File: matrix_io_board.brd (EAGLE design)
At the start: 155.7 x 37.8 mm, 118 parts, among them IC1 6N138, IC10 REG1117, IC12 AP3012, IC2 SN74LVC2G14, IC4 LM324D, IC5 MCP4728_QUAD_DAC, IC6 4504D, IC9 REG1117, J1 1734753-1, Q1 FDN360P

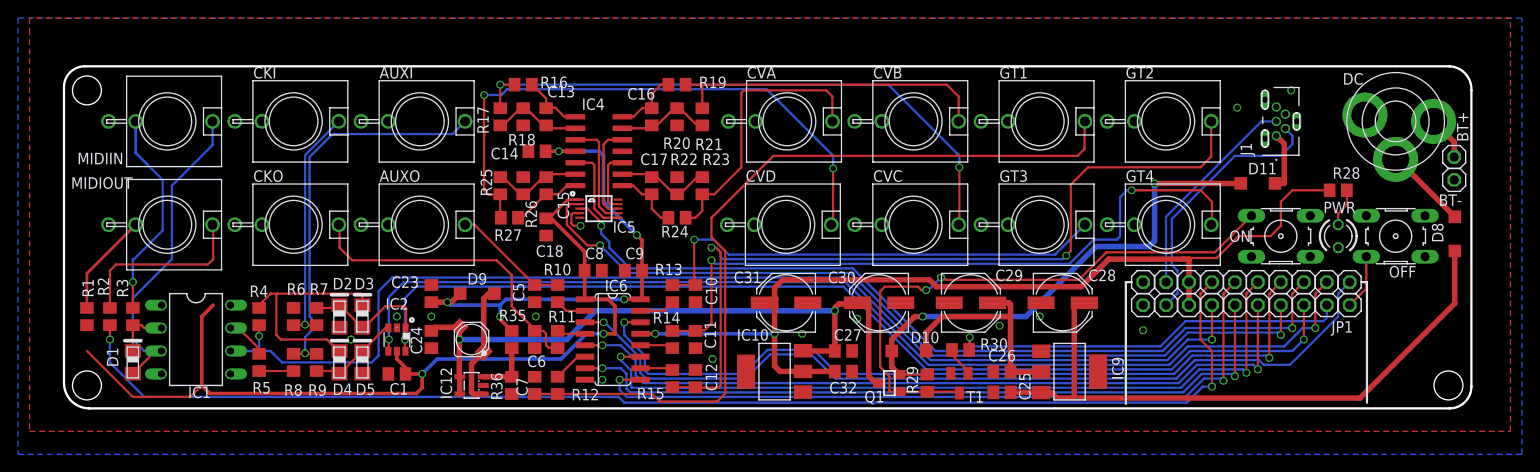
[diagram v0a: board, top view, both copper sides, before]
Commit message: Revert "3v3 updates"
This reverts commit 782c7fb22120100be74f5025aa682998f87b6e62.
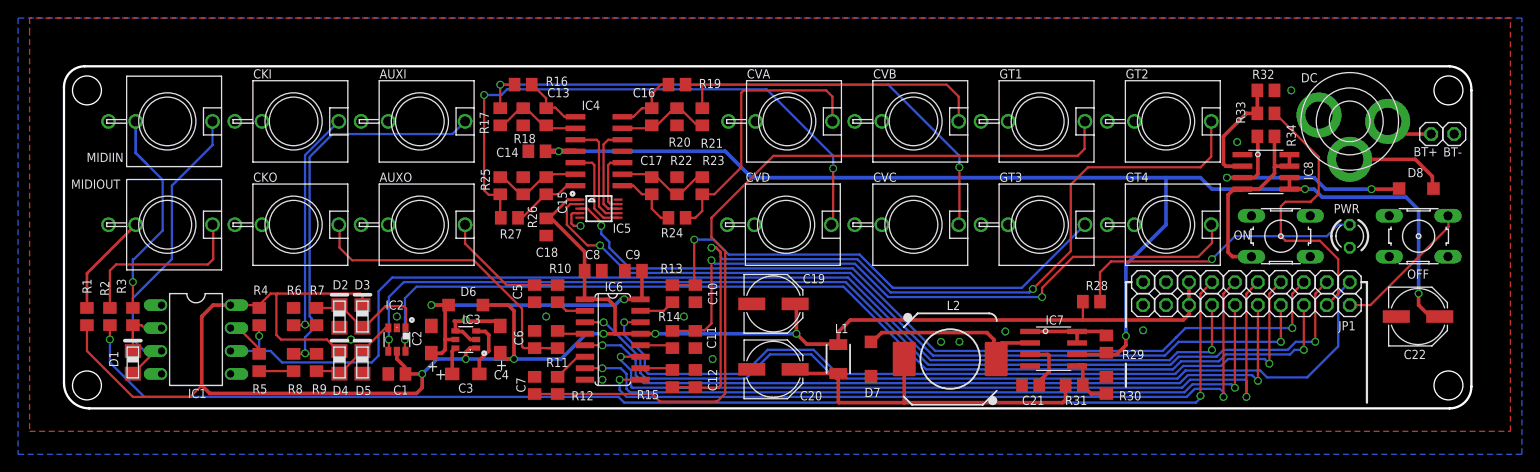
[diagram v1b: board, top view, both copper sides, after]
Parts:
- removed C23, C24: 1u, rcl:C0805
- removed C25, C26, C27, C32: 100n, rcl:C0805
- removed C28, C29, C30, C31: (no value), rcl:PANASONIC_D
- removed D10, D11, D9: MBR0520LT, diode:SOD123
- removed IC10, IC9: REG1117, burr-brown:SOT223
- removed IC12: AP3012, jason2:SOT23-5
- removed J1: 1734753-1, jason2:CONN_1734753-1
- removed Q1: FDN360P, transistor-power:SUPER-SOT3
- removed R35, R36: 1k, rcl:R0805
- removed T1: (no value), transistor:SOT23-BEC
- removed U$2: CDRH3D14, jason2:CDRH3D14
- added C19, C20, C22: (no value), rcl:PANASONIC_D
- added C2, C3, C4: 10u, rcl:SMC_A
- added C21: 470p, rcl:C0805
- added D6, D7: MBR0520LT, diode:SOD123
- added IC3: LM27675M5_CHARGEPUMP, jason_eagle6:SOT23-6
- added IC7: SP34063A_BOOST_REG, jason_eagle6:SOIC8
- added IC8: FDS8958B, jason_eagle6:SOIC8
- added L1: (no value), SparkFun:1210
- added L2: (no value), jason_eagle6:DR1030
- added R31: 3k, rcl:R0805
- added R32, R34: 10k, rcl:R0805
- added R33: 1k, rcl:R0805
- R29: value (none) -> 0r33
- R30: value (none) -> 1k
- moved R28 30.0 mm to (114.9, 13.1)
- moved R29 20.3 mm to (116.6, 8.38)
- moved R30 16.6 mm to (116.6, 3.81), turned to 270 degrees
- moved D8 6.58 mm to (150.9, 25.6), turned to 0 degrees
- moved DC 5.08 mm to (143.5, 33.0)
- moved BT- 5.08 mm to (155.1, 31.6)
- moved BT+ 3.59 mm to (152.5, 31.6)
- moved OFF 2.54 mm to (151.1, 20.3), turned to 0 degrees
- moved PWR 1.27 mm to (143.5, 20.3)
- turned C6 to 270 degrees
- renumbered 3V to 5V, 3V. to 5V., D+ to GD1, D- to GD2
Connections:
- removed net +3V3: 5V..1, 5V.1, C1.1, C18.1, C31.+, C32.2, C8.1, D3.A, D4.A, IC1.8, IC10.2, IC2.5, IC5.1, IC6.1, IC6.13, R1.2, R28.1, R4.2
- removed net N$21: C26.2, C29.+, D10.A, IC9.2
- removed net N$28: D9.A, IC12.1, U$2.1
- removed net N$42: PWRCTL.1, R30.2
- removed net N$52: IC12.3, R35.1, R36.2
- removed net USB_DM: GD2.1, J1.2
- removed net USB_DP: GD1.1, J1.3
- removed net VUSB: D11.A, J1.1
- new net +5V: 5V..1, 5V.1, C1.1, C18.1, C19.+, C4.+, C8.1, D3.A, D4.A, D6.A, IC1.8, IC2.5, IC3.1, IC5.1, IC6.1, IC6.13, L1.2, R1.2, R28.1, R4.2
- new net +9V: C14.1, C22.+, IC4.4, IC7.6, IC8.5, IC8.6, R29.1
- new net N$39: C3.-, IC3.3
- new net N$51: C20.+, L1.1, L2.1, R31.1
- new net N$61: IC8.4, IC8.7, IC8.8, ON.2, R34.2
- new net N$62: IC8.2, R32.2, R33.2
- new net PWR_CTRL: PWRCTL.1, R33.1
- new net VIN: D8.C, IC8.3, R34.1
- net +10V: now also C2.+, D6.C, IC3.5; no longer C14.1, C23.2, D9.C, IC4.4, R35.2
- net GND: now also C19.-, C2.-, C20.-, C21.2, C22.-, C4.-, D7.A, GD1.1, GD2.1, IC3.2, IC3.4, IC7.4, IC8.1, ON.3, R30.1, R32.1; no longer C23.1, C24.1, C25.1, C26.1, C27.1, C28.-, C29.-, C30.-, C31.-, C32.1, IC10.1, IC12.2, IC9.1, J1.5, ON.1, ON.2, R36.1, T1.E
- net N$32: now also IC7.1, IC7.7, IC7.8; no longer D10.C, D11.C, Q1.2
- net N$33: now also IC7.5, R30.2, R31.2; no longer C24.2, C27.2, C30.+, IC10.3, IC12.4, IC12.5, Q1.3, U$2.2
- net N$34: now also C21.1, IC7.3; no longer ON.3, ON.4, Q1.1, R29.1, T1.C
- net N$35: now also D7.C, IC7.2, L2.2; no longer R30.1, T1.B
- net N$38: now also C3.+, IC3.6; no longer C25.2, C28.+, D8.C, IC9.3
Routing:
- net +3V3: track 234.1 -> 0.00 mm, vias 4 -> 0
- net +5V: track 0.00 -> 224.4 mm, vias 0 -> 6
- net +9V: track 0.00 -> 143.9 mm, vias 0 -> 4
- net N$33: track 75.4 -> 6.07 mm, vias 2 -> 0
- net N$38: track 71.1 -> 3.00 mm
- net N$34: track 64.4 -> 5.89 mm, vias 2 -> 0
- net N$32: track 56.9 -> 9.90 mm, vias 2 -> 0
- net N$42: track 44.3 -> 0.00 mm, vias 1 -> 0
- net N$51: track 0.00 -> 39.8 mm
- net PWR_CTRL: track 0.00 -> 32.0 mm
- net USB_DM: track 29.1 -> 0.00 mm
- net N$56: track 4.20 -> 33.0 mm, vias 0 -> 1
- net VIN: track 0.00 -> 27.4 mm, vias 0 -> 2
- net N$21: track 26.2 -> 0.00 mm
- net USB_DP: track 23.8 -> 0.00 mm
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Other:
- board text added: "+"

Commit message: 3v3 updates
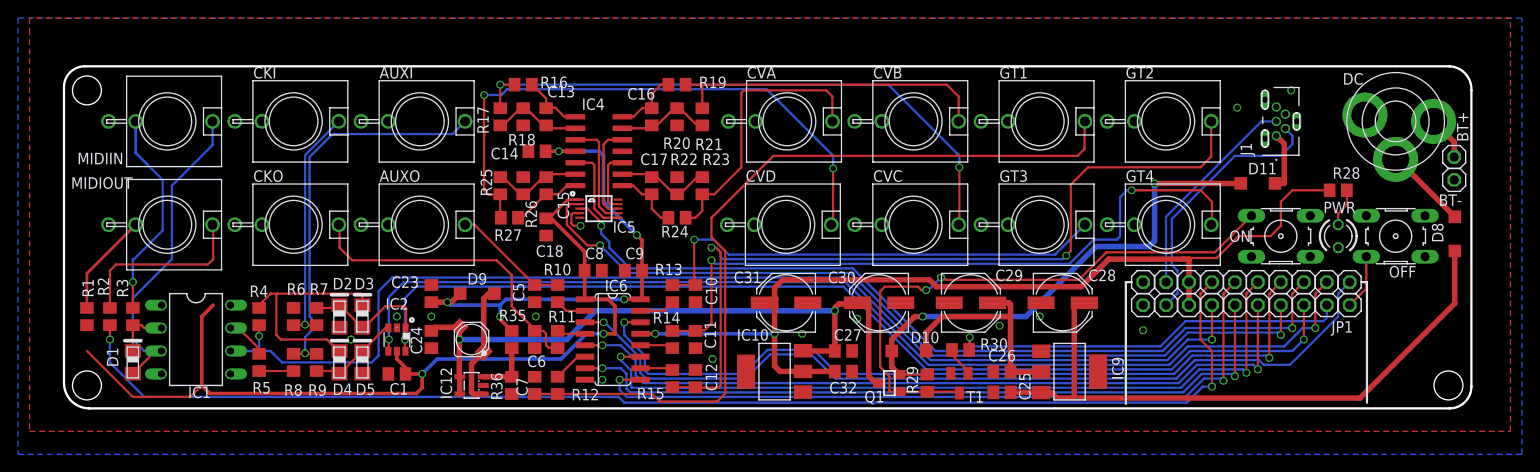
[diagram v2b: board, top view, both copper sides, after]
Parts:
- removed C19, C20, C22: (no value), rcl:PANASONIC_D
- removed C2, C3, C4: 10u, rcl:SMC_A
- removed C21: 470p, rcl:C0805
- removed D6, D7: MBR0520LT, diode:SOD123
- removed IC3: LM27675M5_CHARGEPUMP, jason_eagle6:SOT23-6
- removed IC7: SP34063A_BOOST_REG, jason_eagle6:SOIC8
- removed IC8: FDS8958B, jason_eagle6:SOIC8
- removed L1: (no value), SparkFun:1210
- removed L2: (no value), jason_eagle6:DR1030
- removed R31: 3k, rcl:R0805
- removed R32, R34: 10k, rcl:R0805
- removed R33: 1k, rcl:R0805
- added C23, C24: 1u, rcl:C0805
- added C25, C26, C27, C32: 100n, rcl:C0805
- added C28, C29, C30, C31: (no value), rcl:PANASONIC_D
- added D10, D11, D9: MBR0520LT, diode:SOD123
- added IC10, IC9: REG1117, burr-brown:SOT223
- added IC12: AP3012, jason2:SOT23-5
- added J1: 1734753-1, jason2:CONN_1734753-1
- added Q1: FDN360P, transistor-power:SUPER-SOT3
- added R35, R36: 1k, rcl:R0805
- added T1: (no value), transistor:SOT23-BEC
- added U$2: CDRH3D14, jason2:CDRH3D14
- R29: value 0r33 -> (none)
- R30: value 1k -> (none)
- moved R28 30.0 mm to (142.2, 25.4)
- moved R29 20.3 mm to (96.8, 4.06)
- moved R30 16.6 mm to (100.5, 7.75), turned to 0 degrees
- moved D8 6.58 mm to (155.1, 20.6), turned to 90 degrees
- moved DC 5.08 mm to (148.6, 33.0)
- moved BT- 5.08 mm to (155.1, 26.5)
- moved BT+ 3.59 mm to (155.1, 29.1)
- moved OFF 2.54 mm to (148.6, 20.3), turned to 180 degrees
- moved PWR 1.27 mm to (142.2, 20.3)
- turned C6 to 90 degrees
- renumbered 5V to 3V, 5V. to 3V., GD1 to D+, GD2 to D-
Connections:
- removed net +5V: 3V..1, 3V.1, C1.1, C18.1, C19.+, C4.+, C8.1, D3.A, D4.A, D6.A, IC1.8, IC2.5, IC3.1, IC5.1, IC6.1, IC6.13, L1.2, R1.2, R28.1, R4.2
- removed net +9V: C14.1, C22.+, IC4.4, IC7.6, IC8.5, IC8.6, R29.1
- removed net N$39: C3.-, IC3.3
- removed net N$51: C20.+, L1.1, L2.1, R31.1
- removed net N$61: IC8.4, IC8.7, IC8.8, ON.2, R34.2
- removed net N$62: IC8.2, R32.2, R33.2
- removed net PWR_CTRL: PWRCTL.1, R33.1
- removed net VIN: D8.C, IC8.3, R34.1
- new net +3V3: 3V..1, 3V.1, C1.1, C18.1, C31.+, C32.2, C8.1, D3.A, D4.A, IC1.8, IC10.2, IC2.5, IC5.1, IC6.1, IC6.13, R1.2, R28.1, R4.2
- new net N$21: C26.2, C29.+, D10.A, IC9.2
- new net N$28: D9.A, IC12.1, U$2.1
- new net N$42: PWRCTL.1, R30.2
- new net N$52: IC12.3, R35.1, R36.2
- new net USB_DM: D-.1, J1.2
- new net USB_DP: D+.1, J1.3
- new net VUSB: D11.A, J1.1
- net +10V: now also C14.1, C23.2, D9.C, IC4.4, R35.2; no longer C2.+, D6.C, IC3.5
- net GND: now also C23.1, C24.1, C25.1, C26.1, C27.1, C28.-, C29.-, C30.-, C31.-, C32.1, IC10.1, IC12.2, IC9.1, J1.5, ON.1, ON.2, R36.1, T1.E; no longer C19.-, C2.-, C20.-, C21.2, C22.-, C4.-, D+.1, D-.1, D7.A, IC3.2, IC3.4, IC7.4, IC8.1, ON.3, R30.1, R32.1
- net N$32: now also D10.C, D11.C, Q1.2; no longer IC7.1, IC7.7, IC7.8
- net N$33: now also C24.2, C27.2, C30.+, IC10.3, IC12.4, IC12.5, Q1.3, U$2.2; no longer IC7.5, R30.2, R31.2
- net N$34: now also ON.3, ON.4, Q1.1, R29.1, T1.C; no longer C21.1, IC7.3
- net N$35: now also R30.1, T1.B; no longer D7.C, IC7.2, L2.2
- net N$38: now also C25.2, C28.+, D8.C, IC9.3; no longer C3.+, IC3.6
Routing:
- net +3V3: track 0.00 -> 234.1 mm, vias 0 -> 4
- net +5V: track 224.4 -> 0.00 mm, vias 6 -> 0
- net +9V: track 143.9 -> 0.00 mm, vias 4 -> 0
- net N$33: track 6.07 -> 75.4 mm, vias 0 -> 2
- net N$38: track 3.00 -> 71.1 mm
- net N$34: track 5.89 -> 64.4 mm, vias 0 -> 2
- net N$32: track 9.90 -> 56.9 mm, vias 0 -> 2
- net N$42: track 0.00 -> 44.3 mm, vias 0 -> 1
- net N$51: track 39.8 -> 0.00 mm
- net PWR_CTRL: track 32.0 -> 0.00 mm
- net USB_DM: track 0.00 -> 29.1 mm
- net N$56: track 33.0 -> 4.20 mm, vias 1 -> 0
- net VIN: track 27.4 -> 0.00 mm, vias 2 -> 0
- net N$21: track 0.00 -> 26.2 mm
- net USB_DP: track 0.00 -> 23.8 mm
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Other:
- board text removed: "+"
